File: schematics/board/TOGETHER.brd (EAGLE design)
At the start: 22 x 22 mm, 12 parts

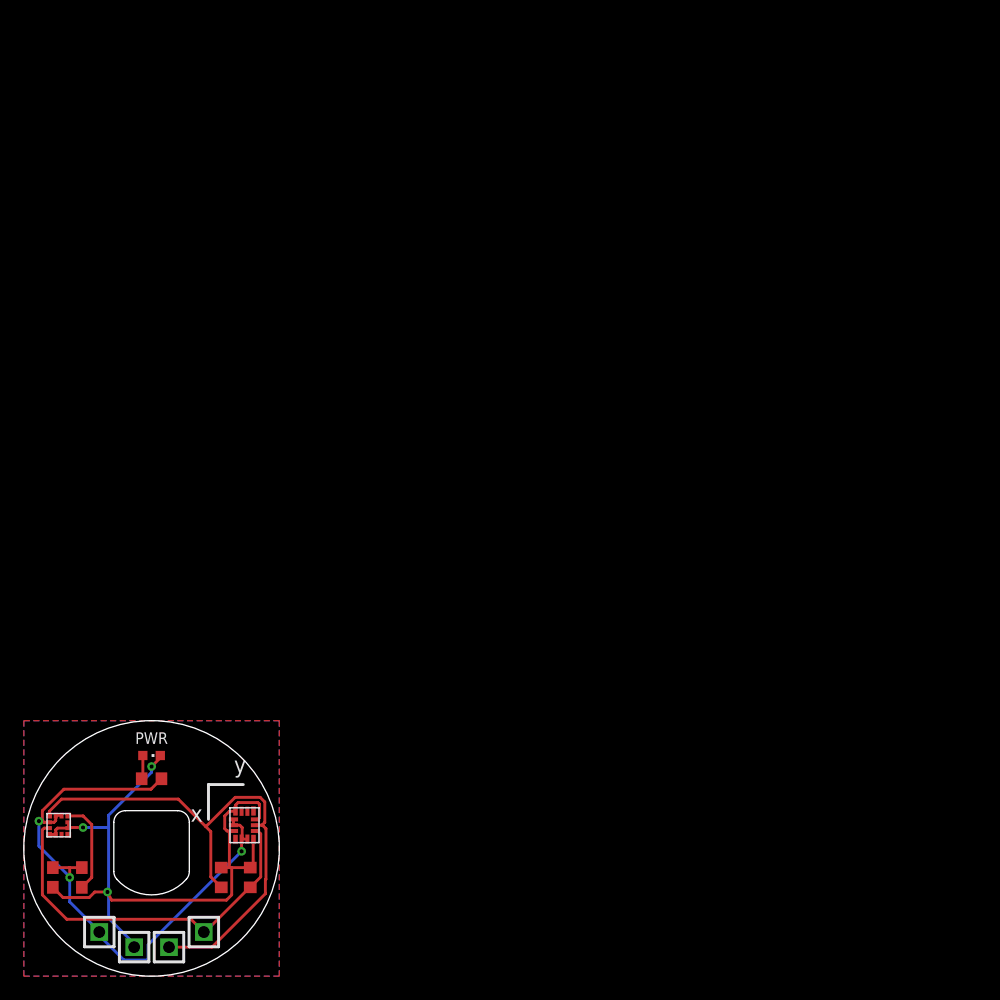
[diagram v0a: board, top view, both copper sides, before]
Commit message: Добавлена плата TOGETHER
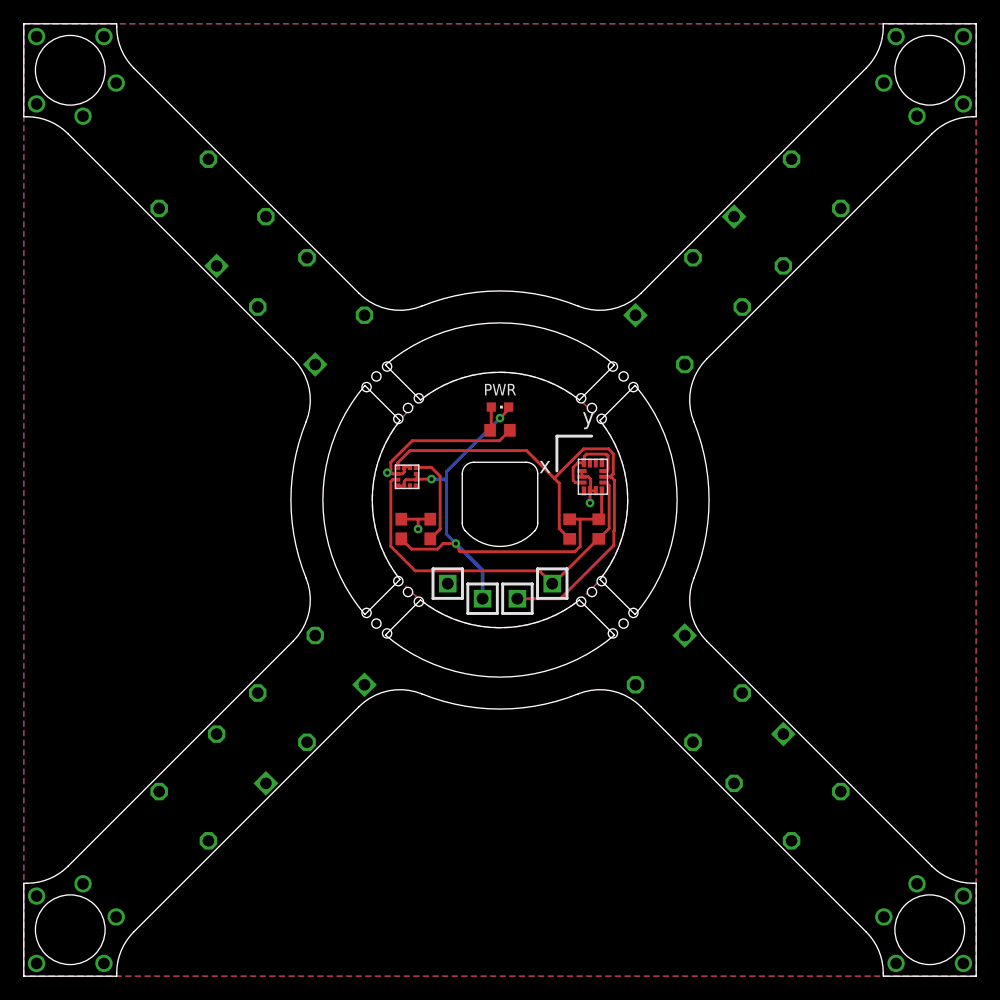
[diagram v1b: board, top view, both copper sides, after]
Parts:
- added U$1, U$18, U$19, U$2, U$20, U$21, U$3, U$4: KCONNECT-, CanCubeSat:KCONNECT-
- moved 3V3 42.4 mm to (39.5, 32.5)
- moved C1 42.4 mm to (32.5, 38.5)
- moved C10 42.4 mm to (35.0, 38.5)
- moved LIS3MDL 42.4 mm to (33.0, 43.0)
- moved LSM6DS3 42.4 mm to (49.0, 43.0)
- moved PWR 42.4 mm to (41.0, 49.0)
- moved R1 42.4 mm to (41.0, 47.0)
- moved R101 42.4 mm to (47.0, 38.5)
- moved R102 42.4 mm to (49.5, 38.5)
- moved SCL 42.4 mm to (42.5, 32.5)
- moved GND 42.4 mm to (36.5, 33.8)
- moved SDA 42.4 mm to (45.5, 33.8)
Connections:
- net GND renamed GND1
- new net BUS+: U$1.1, U$1.2, U$1.3, U$1.4, U$18.1, U$18.2, U$18.3, U$18.4, U$20.1, U$20.2, U$20.3, U$20.4, U$3.1, U$3.2, U$3.3, U$3.4
- new net BUS-: U$19.1, U$19.2, U$19.3, U$19.4, U$2.1, U$2.2, U$2.3, U$2.4, U$21.1, U$21.2, U$21.3, U$21.4, U$4.1, U$4.2, U$4.3, U$4.4
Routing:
- net GND1: track 51.8 -> 22.0 mm
- net VDD: track 59.9 -> 56.7 mm
- added copper zone on layer 16, net BUS+
- added copper zone on layer 1, net BUS-
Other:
- board size 22 x 22 mm -> 82 x 82 mm
